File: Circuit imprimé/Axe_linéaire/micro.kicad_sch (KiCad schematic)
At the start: 8 parts, among them Q1 LP2301LT1G, SW1 RESET, U1 PicoW

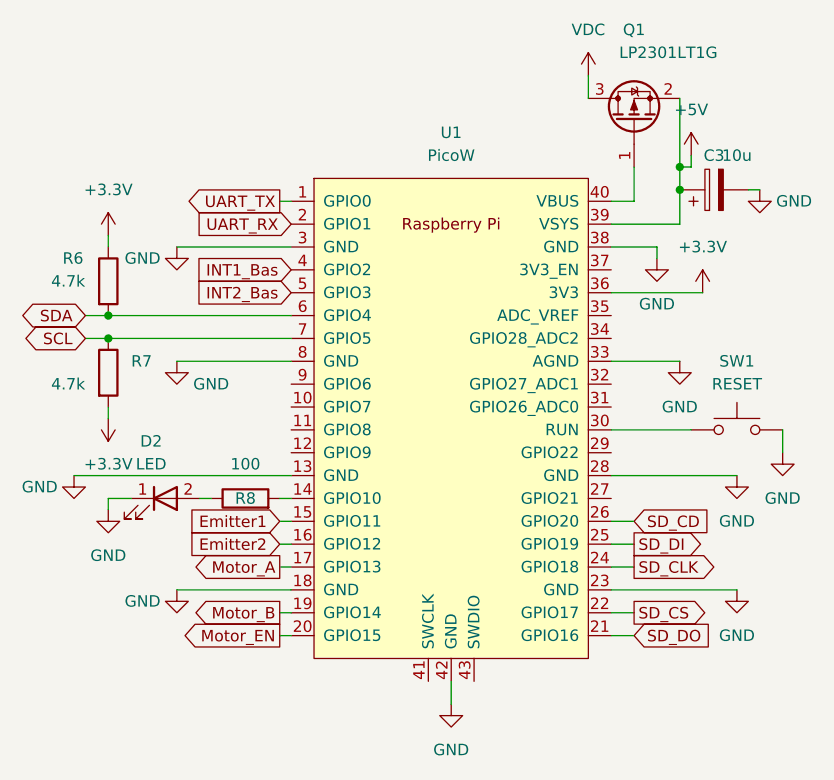
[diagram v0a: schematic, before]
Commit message: circuit V1
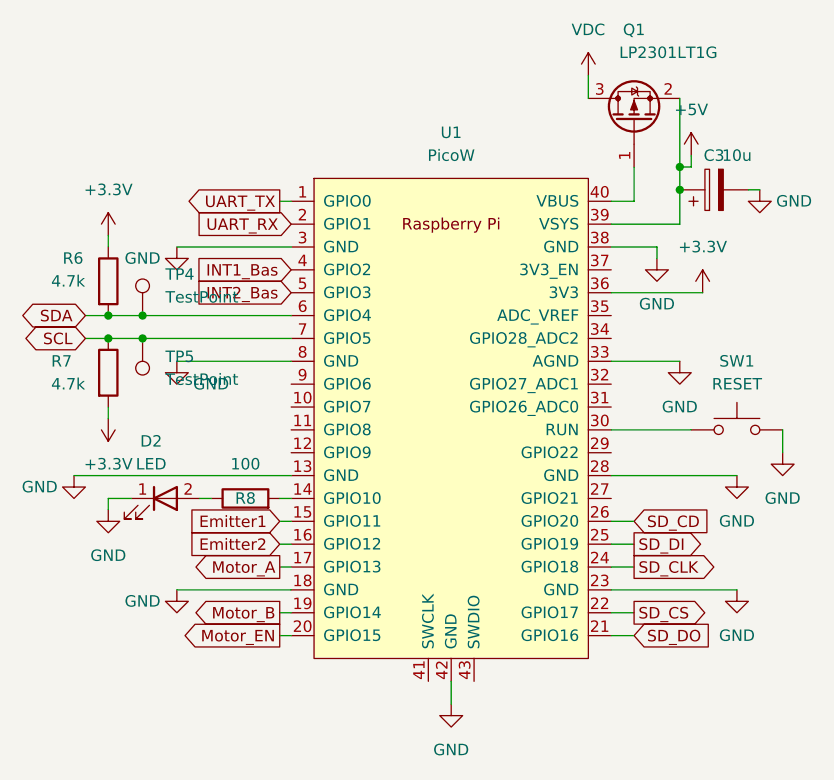
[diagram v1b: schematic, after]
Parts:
- added TP4, TP5: TestPoint, TestPoint:TestPoint_Pad_D2.0mm, symbol Connector:TestPoint
- C3: footprint (none) -> Capacitor_SMD:CP_Elec_6.3x7.7
- R6, R7, R8: footprint (none) -> Resistor_SMD:R_0603_1608Metric
- U1: footprint RPi_PicoW:RPi_Pico_SMD_TH -> RPi_Pico:RPi_PicoW_SMD_TH
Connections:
- net SCL: now also TP5.1
- net SDA: now also TP4.1
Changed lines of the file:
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@@
   (junction (at 166.37 40.64) (diameter 0) (color 0 0 0 0)
   )
+  (junction (at 106.68 57.15) (diameter 0) (color 0 0 0 0)
+  )
   (junction (at 166.37 43.18) (diameter 0) (color 0 0 0 0)
   )
   (junction (at 102.87 59.69) (diameter 0) (color 0 0 0 0)
   )
+  (junction (at 106.68 59.69) (diameter 0) (color 0 0 0 0)
+  )
   (wire (pts (xy 158.75 85.09) (xy 161.29 85.09))
     (stroke (width 0) (type default) (color 0 0 0 0))
@@
     (stroke (width 0) (type default) (color 0 0 0 0))
   )
-  (wire (pts (xy 102.87 59.69) (xy 123.19 59.69))
+  (wire (pts (xy 102.87 59.69) (xy 106.68 59.69))
     (stroke (width 0) (type default) (color 0 0 0 0))
   )
@@
     (stroke (width 0) (type default) (color 0 0 0 0))
   )
+  (wire (pts (xy 106.68 59.69) (xy 123.19 59.69))
+    (stroke (width 0) (type default) (color 0 0 0 0))
+  )
   (wire (pts (xy 158.75 54.61) (xy 168.91 54.61))
     (stroke (width 0) (type default) (color 0 0 0 0))
@@
     (stroke (width 0) (type default) (color 0 0 0 0))
   )
-  (wire (pts (xy 102.87 57.15) (xy 123.19 57.15))
+  (wire (pts (xy 102.87 57.15) (xy 106.68 57.15))
     (stroke (width 0) (type default) (color 0 0 0 0))
   )
@@
   )
   (wire (pts (xy 158.75 49.53) (xy 163.83 49.53))
+    (stroke (width 0) (type default) (color 0 0 0 0))
+  )
+  (wire (pts (xy 106.68 57.15) (xy 123.19 57.15))
     (stroke (width 0) (type default) (color 0 0 0 0))
   )
@@
     (property "Reference" "R8" (id 0) (at 118.11 77.47 90))
     (property "Value" "100" (id 1) (at 118.11 73.66 90))
-    (property "Footprint" "" (id 2) (at 118.11 79.248 90)
+    (property "Footprint" "Resistor_SMD:R_0603_1608Metric" (id 2) (at 118.11 79.248 90)
       (effects (font (size 1.27 1.27)) hide)
     )
@@
   (symbol (lib_id "Device:R") (at 102.87 63.5 0) (unit 1)
     (in_bom yes) (on_board yes)
-    (property "Reference" "R7" (id 0) (at 105.41 62.2299 0)
+    (property "Reference" "R7" (id 0) (at 96.52 62.23 0)
       (effects (font (size 1.27 1.27)) (justify left))
     )
@@
       (effects (font (size 1.27 1.27)) (justify left))
     )
-    (property "Footprint" "" (id 2) (at 101.092 63.5 90)
+    (property "Footprint" "Resistor_SMD:R_0603_1608Metric" (id 2) (at 101.092 63.5 90)
       (effects (font (size 1.27 1.27)) hide)
     )
@@
     (property "Reference" "C3" (id 0) (at 170.18 39.37 90))
     (property "Value" "10u" (id 1) (at 172.72 39.37 90))
-    (property "Footprint" "" (id 2) (at 173.99 42.2148 0)
+    (property "Footprint" "Capacitor_SMD:CP_Elec_6.3x7.7" (id 2) (at 173.99 42.2148 0)
       (effects (font (size 1.27 1.27)) hide)
     )
@@
     (property "Reference" "U1" (id 0) (at 140.97 36.83 0))
     (property "Value" "PicoW" (id 1) (at 140.97 39.37 0))
-    (property "Footprint" "RPi_PicoW:RPi_Pico_SMD_TH" (id 2) (at 140.97 68.58 90)
+    (property "Footprint" "RPi_Pico:RPi_PicoW_SMD_TH" (id 2) (at 140.97 68.58 90)
       (effects (font (size 1.27 1.27)) hide)
     )
@@
     (pin "1")
   )
+  (symbol (lib_id "Connector:TestPoint") (at 106.68 59.69 180) (unit 1)
+    (in_bom yes) (on_board yes) (fields_autoplaced)
+    (property "Reference" "TP5" (id 0) (at 109.22 61.7219 0)
+      (effects (font (size 1.27 1.27)) (justify right))
+    )
+    (property "Value" "TestPoint" (id 1) (at 109.22 64.2619 0)
+      (effects (font (size 1.27 1.27)) (justify right))
+    )
+    (property "Footprint" "TestPoint:TestPoint_Pad_D2.0mm" (id 2) (at 101.6 59.69 0)
+      (effects (font (size 1.27 1.27)) hide)
+    )
+    (property "Datasheet" "~" (id 3) (at 101.6 59.69 0)
+      (effects (font (size 1.27 1.27)) hide)
+    )
+    (pin "1")
+  )
   (symbol (lib_id "power:GND") (at 175.26 43.18 0) (unit 1)
     (in_bom yes) (on_board yes)
@@
       (effects (font (size 1.27 1.27)) (justify left))
     )
-    (property "Footprint" "" (id 2) (at 101.092 53.34 90)
+    (property "Footprint" "Resistor_SMD:R_0603_1608Metric" (id 2) (at 101.092 53.34 90)
       (effects (font (size 1.27 1.27)) hide)
     )
@@
       (effects (font (size 1.27 1.27)) hide)
     )
+    (pin "1")
+  )
+  (symbol (lib_id "Connector:TestPoint") (at 106.68 57.15 0) (unit 1)
+    (in_bom yes) (on_board yes) (fields_autoplaced)
+    (property "Reference" "TP4" (id 0) (at 109.22 52.5779 0)
+      (effects (font (size 1.27 1.27)) (justify left))
+    )
+    (property "Value" "TestPoint" (id 1) (at 109.22 55.1179 0)
+      (effects (font (size 1.27 1.27)) (justify left))
+    )
+    (property "Footprint" "TestPoint:TestPoint_Pad_D2.0mm" (id 2) (at 111.76 57.15 0)
+      (effects (font (size 1.27 1.27)) hide)
+    )
+    (property "Datasheet" "~" (id 3) (at 111.76 57.15 0)
+      (effects (font (size 1.27 1.27)) hide)
+    )

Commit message: tout mes CI sont pret
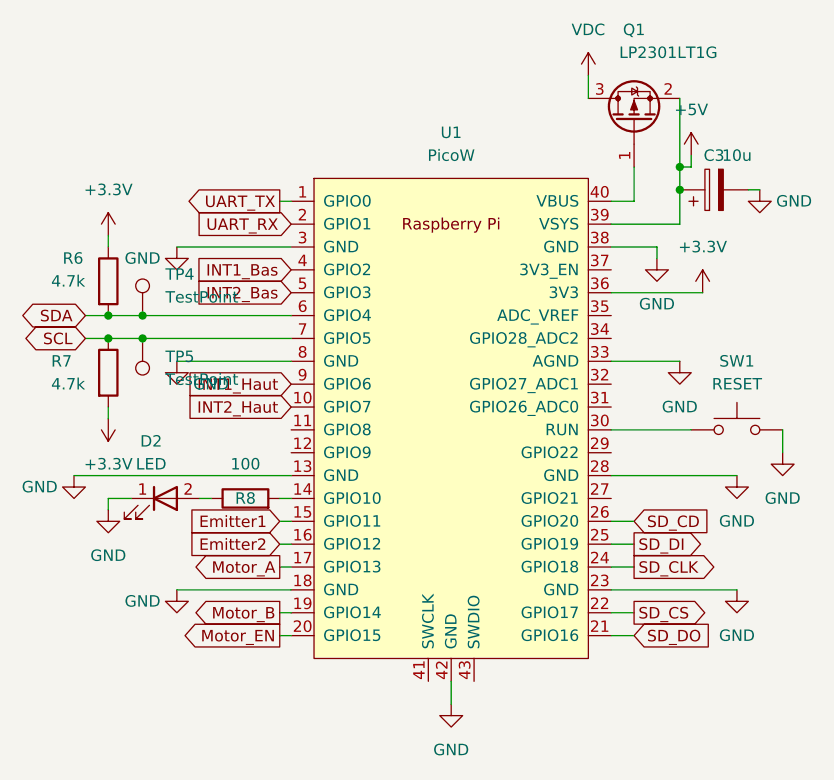
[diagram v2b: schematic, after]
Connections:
- net INT2_Haut: now reaches U1.10 (GPIO7)
- net INT1_Haut: now reaches U1.9 (GPIO6)
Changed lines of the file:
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@@
+    )
+  )
+  (global_label "INT2_Haut" (shape input) (at 123.19 67.31 180) (fields_autoplaced)
+    (effects (font (size 1.27 1.27)) (justify right))
+    (property "Intersheet References" "${INTERSHEET_REFS}" (id 0) (at 111.3426 67.2306 0)
+      (effects (font (size 1.27 1.27)) (justify right) hide)
     )
   )
@@
     )
   )
+  (global_label "INT1_Haut" (shape input) (at 123.19 64.77 180) (fields_autoplaced)
+    (effects (font (size 1.27 1.27)) (justify right))
+    (property "Intersheet References" "${INTERSHEET_REFS}" (id 0) (at 111.3426 64.6906 0)
+      (effects (font (size 1.27 1.27)) (justify right) hide)
+    )
+  )
